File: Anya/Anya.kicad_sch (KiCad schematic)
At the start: 76 parts, among them SW1 SW_Push, SW10 SW_Push, SW11 SW_Push, SW12 SW_Push, SW13 SW_Push, SW14 SW_Push, SW15 SW_Push, SW16 SW_Push, SW17 SW_Push, SW18 SW_Push, SW19 SW_Push, SW2 SW_Push, SW20 SW_Push, SW21 SW_Push, SW22 SW_Push, SW23 SW_Push, SW24 SW_Push, SW25 SW_Push, SW26 SW_Push, SW27 SW_Push, SW28 SW_Push, SW29 SW_Push, SW3 SW_Push, SW30 SW_Push, SW31 SW_Push, SW32 SW_Push, SW33 SW_Push, SW4 SW_Push, SW5 SW_Push, SW6 SW_Push, SW7 SW_Push, SW8 SW_Push, SW9 SW_Push, U1 ProMicro

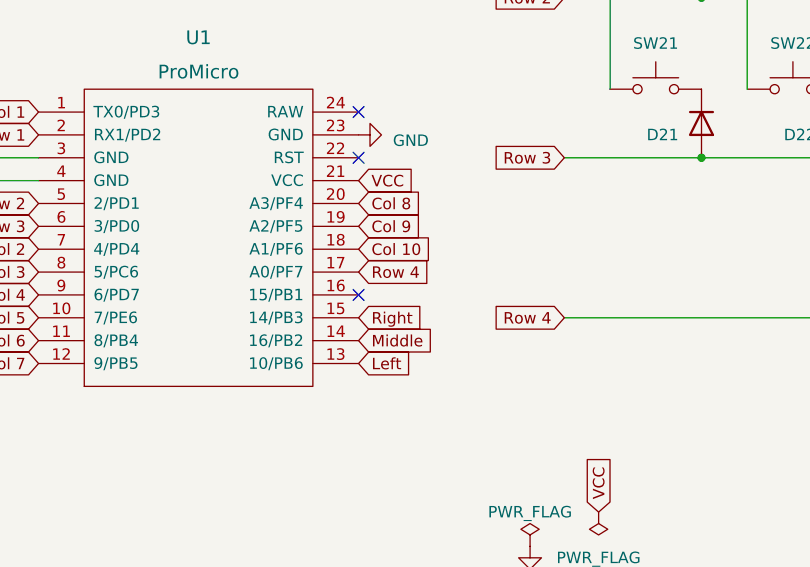
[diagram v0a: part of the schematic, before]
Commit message: Anya R1
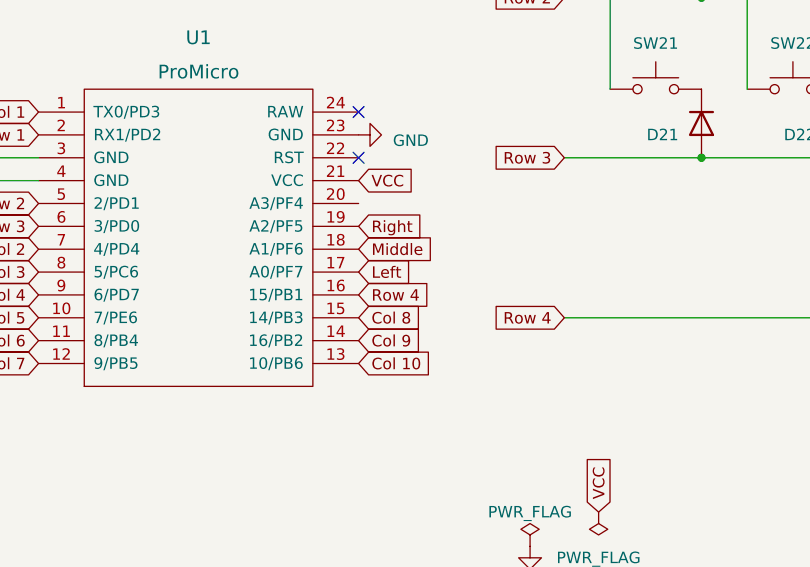
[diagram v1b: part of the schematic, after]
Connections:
- net Col 10: now also U1.13 (10/PB6); no longer U1.18 (A1/PF6)
- net Col 8: now also U1.15 (14/PB3); no longer U1.20 (A3/PF4)
- net Col 9: now also U1.14 (16/PB2); no longer U1.19 (A2/PF5)
- net Left: now also U1.17 (A0/PF7); no longer U1.13 (10/PB6)
- net Middle: now also U1.18 (A1/PF6); no longer U1.14 (16/PB2)
- net Right: now also U1.19 (A2/PF5); no longer U1.15 (14/PB3)
- net Row 4: now also U1.16 (15/PB1); no longer U1.17 (A0/PF7)
- no-connect marks 3 -> 2
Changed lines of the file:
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@@
   )
   (no_connect (at 73.66 119.38))
-  (no_connect (at 73.66 134.62))
   (no_connect (at 73.66 114.3))
   (wire (pts (xy 233.68 83.82) (xy 248.92 83.82))
@@
     )
   )
-  (global_label "Col 10" (shape input) (at 73.66 129.54 0) (fields_autoplaced)
-    (effects (font (size 1.27 1.27)) (justify left))
-    (property "Intersheetrefs" "${INTERSHEET_REFS}" (at 83.0366 129.54 0)
-      (effects (font (size 1.27 1.27)) (justify left) hide)
-    )
-  )
-  (global_label "Right" (shape input) (at 73.66 137.16 0) (fields_autoplaced)
-    (effects (font (size 1.27 1.27)) (justify left))
-    (property "Intersheetrefs" "${INTERSHEET_REFS}" (at 81.4643 137.16 0)
+  (global_label "Col 10" (shape input) (at 73.66 142.24 0) (fields_autoplaced)
+    (effects (font (size 1.27 1.27)) (justify left))
+    (property "Intersheetrefs" "${INTERSHEET_REFS}" (at 83.0366 142.24 0)
+      (effects (font (size 1.27 1.27)) (justify left) hide)
+    )
+  )
+  (global_label "Right" (shape input) (at 73.66 127 0) (fields_autoplaced)
+    (effects (font (size 1.27 1.27)) (justify left))
+    (property "Intersheetrefs" "${INTERSHEET_REFS}" (at 81.4643 127 0)
       (effects (font (size 1.27 1.27)) (justify left) hide)
     )
@@
     )
   )
-  (global_label "Middle" (shape input) (at 73.66 139.7 0) (fields_autoplaced)
-    (effects (font (size 1.27 1.27)) (justify left))
-    (property "Intersheetrefs" "${INTERSHEET_REFS}" (at 82.6738 139.7 0)
+  (global_label "Middle" (shape input) (at 73.66 129.54 0) (fields_autoplaced)
+    (effects (font (size 1.27 1.27)) (justify left))
+    (property "Intersheetrefs" "${INTERSHEET_REFS}" (at 82.6738 129.54 0)
       (effects (font (size 1.27 1.27)) (justify left) hide)
     )
@@
     )
   )
-  (global_label "Col 8" (shape input) (at 73.66 124.46 0) (fields_autoplaced)
-    (effects (font (size 1.27 1.27)) (justify left))
-    (property "Intersheetrefs" "${INTERSHEET_REFS}" (at 81.8271 124.46 0)
+  (global_label "Col 8" (shape input) (at 73.66 137.16 0) (fields_autoplaced)
+    (effects (font (size 1.27 1.27)) (justify left))
+    (property "Intersheetrefs" "${INTERSHEET_REFS}" (at 81.8271 137.16 0)
       (effects (font (size 1.27 1.27)) (justify left) hide)
     )
@@
     )
   )
-  (global_label "Row 4" (shape input) (at 73.66 132.08 0) (fields_autoplaced)
-    (effects (font (size 1.27 1.27)) (justify left))
-    (property "Intersheetrefs" "${INTERSHEET_REFS}" (at 82.4924 132.08 0)
+  (global_label "Row 4" (shape input) (at 73.66 134.62 0) (fields_autoplaced)
+    (effects (font (size 1.27 1.27)) (justify left))
+    (property "Intersheetrefs" "${INTERSHEET_REFS}" (at 82.4924 134.62 0)
       (effects (font (size 1.27 1.27)) (justify left) hide)
     )
@@
     )
   )
-  (global_label "Left" (shape input) (at 73.66 142.24 0) (fields_autoplaced)
-    (effects (font (size 1.27 1.27)) (justify left))
-    (property "Intersheetrefs" "${INTERSHEET_REFS}" (at 80.1339 142.24 0)
+  (global_label "Left" (shape input) (at 73.66 132.08 0) (fields_autoplaced)
+    (effects (font (size 1.27 1.27)) (justify left))
+    (property "Intersheetrefs" "${INTERSHEET_REFS}" (at 80.1339 132.08 0)
       (effects (font (size 1.27 1.27)) (justify left) hide)
     )
@@
     )
   )
-  (global_label "Col 9" (shape input) (at 73.66 127 0) (fields_autoplaced)
-    (effects (font (size 1.27 1.27)) (justify left))
-    (property "Intersheetrefs" "${INTERSHEET_REFS}" (at 81.8271 127 0)
-      (effects (font (size 1.27 1.27)) (justify left) hide)
-    )
+  (global_label "Col 9" (shape input) (at 73.66 139.7 0) (fields_autoplaced)
+    (effects (font (size 1.27 1.27)) (justify left))
+    (property "Intersheetrefs" "${INTERSHEET_REFS}" (at 81.8271 139.7 0)
+      (effects (font (size 1.27 1.27)) (justify left) hide)
+    )
